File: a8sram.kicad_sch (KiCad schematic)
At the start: 8 parts, among them J1 D, U1 GAL16V8, U5 KM62256CLP, U6 KM62256CLP

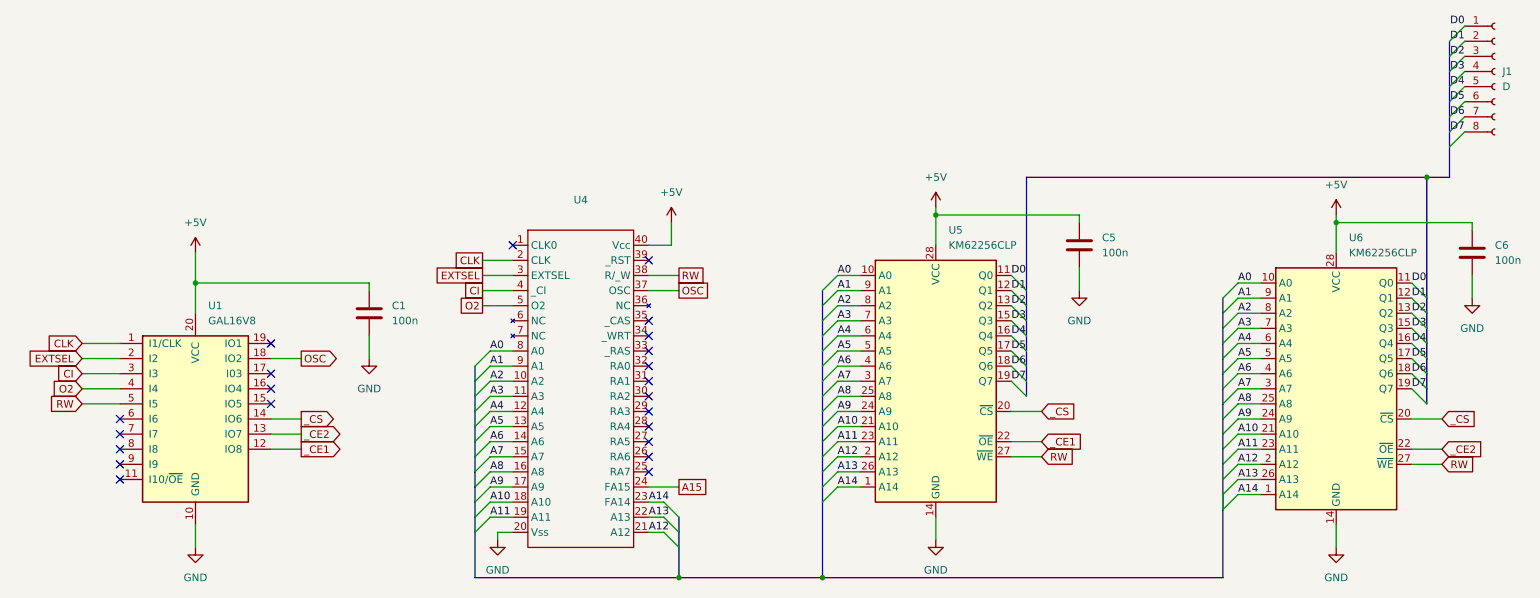
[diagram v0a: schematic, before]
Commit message: wip
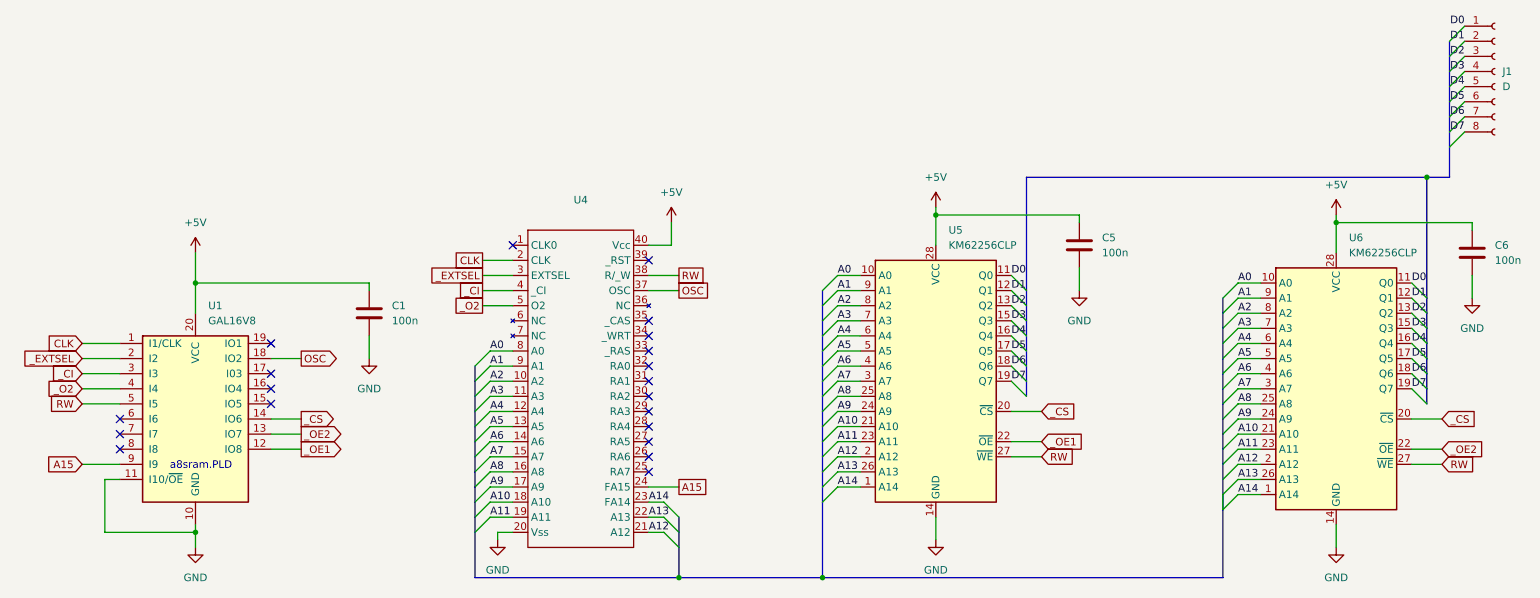
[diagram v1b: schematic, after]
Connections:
- net A15: now also U1.9 (I9)
- net GND: now also U1.11 (I10/~{OE})
- net CI renamed _CI
- net EXTSEL renamed _EXTSEL
- net O2 renamed _O2
- net _CE1 renamed _OE1
- net _CE2 renamed _OE2
- no-connect marks 22 -> 20
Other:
- note added: "a8sram.PLD"
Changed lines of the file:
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@@
 	(generator_version "9.0")
 	(paper "A4")
+	(text "a8sram.PLD"
+		(exclude_from_sim no)
+		(at 56.642 118.364 0)
+		(effects
+			(font
+				(size 1.27 1.27)
+			)
+			(justify left)
+			(href "file://a8sram.pld")
+		)
+	)
 	(junction
 		(at 267.97 69.85)
@@
 	)
 	(junction
+		(at 60.96 129.54)
+		(diameter 0)
+		(color 0 0 0 0)
+	)
+	(junction
 		(at 166.37 137.16)
 		(diameter 0)
@@
 	)
 	(no_connect
-		(at 48.26 118.11)
-	)
-	(no_connect
 		(at 137.16 99.06)
 	)
@@
 	)
 	(no_connect
-		(at 48.26 120.65)
-	)
-	(no_connect
 		(at 114.3 81.28)
 	)
@@
 		)
 	)
+	(wire
+		(pts
+			(xy 41.91 118.11) (xy 48.26 118.11)
+		)
+		(stroke
+			(width 0)
+			(type default)
+		)
+	)
 	(bus
 		(pts
@@
 		)
 	)
+	(wire
+		(pts
+			(xy 60.96 129.54) (xy 60.96 132.08)
+		)
+		(stroke
+			(width 0)
+			(type default)
+		)
+	)
 	(bus
 		(pts
@@
 	(wire
 		(pts
+			(xy 45.72 129.54) (xy 60.96 129.54)
+		)
+		(stroke
+			(width 0)
+			(type default)
+		)
+	)
+	(wire
+		(pts
+			(xy 48.26 120.65) (xy 45.72 120.65)
+		)
+		(stroke
+			(width 0)
+			(type default)
+		)
+	)
+	(wire
+		(pts
 			(xy 73.66 113.03) (xy 78.74 113.03)
 		)
@@
 	(wire
 		(pts
-			(xy 60.96 128.27) (xy 60.96 132.08)
+			(xy 60.96 128.27) (xy 60.96 129.54)
 		)
 		(stroke
@@
 	(wire
 		(pts
+			(xy 45.72 120.65) (xy 45.72 129.54)
+		)
+		(stroke
+			(width 0)
+			(type default)
+		)
+	)
+	(wire
+		(pts
 			(xy 168.91 116.84) (xy 172.72 116.84)
 		)
@@
 		)
 	)
-	(global_label "_CE2"
+	(global_label "_OE2"
 		(shape input)
 		(at 270.51 115.57 0)
@@
 		)
 		(property "Intersheetrefs" "${INTERSHEET_REFS}"
-			(at 278.0913 115.57 0)
+			(at 278.1518 115.57 0)
 			(effects
 				(font
@@
 		)
 	)
-	(global_label "CI"
+	(global_label "_CI"
 		(shape input)
 		(at 41.91 102.87 180)
@@
 		)
 		(property "Intersheetrefs" "${INTERSHEET_REFS}"
-			(at 37.05 102.87 0)
+			(at 36.0824 102.87 0)
 			(effects
 				(font
@@
 		)
 	)
-	(global_label "O2"
+	(global_label "_O2"
 		(shape passive)
 		(at 109.22 91.44 180)
@@
 		)
 		(property "Intersheetrefs" "${INTERSHEET_REFS}"
-			(at 104.8061 91.44 0)
+			(at 103.8385 91.44 0)
 			(effects
 				(font
@@
 		)
 	)
-	(global_label "CI"
+	(global_label "_CI"
 		(shape passive)
 		(at 109.22 88.9 180)
@@
 		)
 		(property "Intersheetrefs" "${INTERSHEET_REFS}"
-			(at 105.4713 88.9 0)
+			(at 104.5037 88.9 0)
 			(effects
 				(font
@@
 		)
 	)
-	(global_label "EXTSEL"
+	(global_label "_EXTSEL"
 		(shape passive)
 		(at 109.22 86.36 180)
@@
 		)
 		(property "Intersheetrefs" "${INTERSHEET_REFS}"
-			(at 100.6334 86.36 0)
+			(at 99.6658 86.36 0)
 			(effects
 				(font
@@
 		)
 	)
-	(global_label "O2"
+	(global_label "_O2"
 		(shape input)
 		(at 41.91 105.41 180)
@@
 		)
 		(property "Intersheetrefs" "${INTERSHEET_REFS}"
-			(at 36.3848 105.41 0)
+			(at 35.4172 105.41 0)
 			(effects
 				(font
@@
 		)
 	)
-	(global_label "_CE1"
+	(global_label "_OE1"
 		(shape output)
 		(at 78.74 115.57 0)
@@
 		)
 		(property "Intersheetrefs" "${INTERSHEET_REFS}"
-			(at 86.3213 115.57 0)
+			(at 86.3818 115.57 0)
 			(effects
 				(font
@@
 		)
 	)
-	(global_label "_CE2"
+	(global_label "_OE2"
 		(shape output)
 		(at 78.74 113.03 0)
@@
 		)
 		(property "Intersheetrefs" "${INTERSHEET_REFS}"
-			(at 86.3213 113.03 0)
+			(at 86.3818 113.03 0)
 			(effects
 				(font
@@
 		)
 	)
-	(global_label "_CE1"
+	(global_label "A15"
+		(shape input)
+		(at 41.91 118.11 180)
+		(fields_autoplaced yes)
+		(effects
+			(font
+				(size 1.27 1.27)
+			)
+			(justify right)
+		)
+		(property "Intersheetrefs" "${INTERSHEET_REFS}"
+			(at 35.4172 118.11 0)
+			(effects
+				(font
+					(size 1.27 1.27)
+				)
+				(justify right)
+				(hide yes)
+			)
+		)
+	)
+	(global_label "_OE1"
 		(shape input)
 		(at 203.2 114.3 0)
@@
 		)
 		(property "Intersheetrefs" "${INTERSHEET_REFS}"
-			(at 210.7813 114.3 0)
+			(at 210.8418 114.3 0)
 			(effects
 				(font
@@
 		)
 	)
-	(global_label "EXTSEL"
+	(global_label "_EXTSEL"
 		(shape input)
 		(at 41.91 100.33 180)
@@
 		)
 		(property "Intersheetrefs" "${INTERSHEET_REFS}"
-			(at 32.2121 100.33 0)
+			(at 31.2445 100.33 0)
 			(effects
 				(font
